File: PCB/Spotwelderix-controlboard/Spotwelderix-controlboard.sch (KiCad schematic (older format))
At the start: 45 parts, among them J1 LEDs, J2 ChargerPower, J3 ExtPwr_FAn, J4 Testpin, P1 Display, P2 CONN_01X08, Q1 AO3400A, Q2 AO3400A, Q3 AO3400A, U1 NodeMCU32, U2 LM7805M_TO263

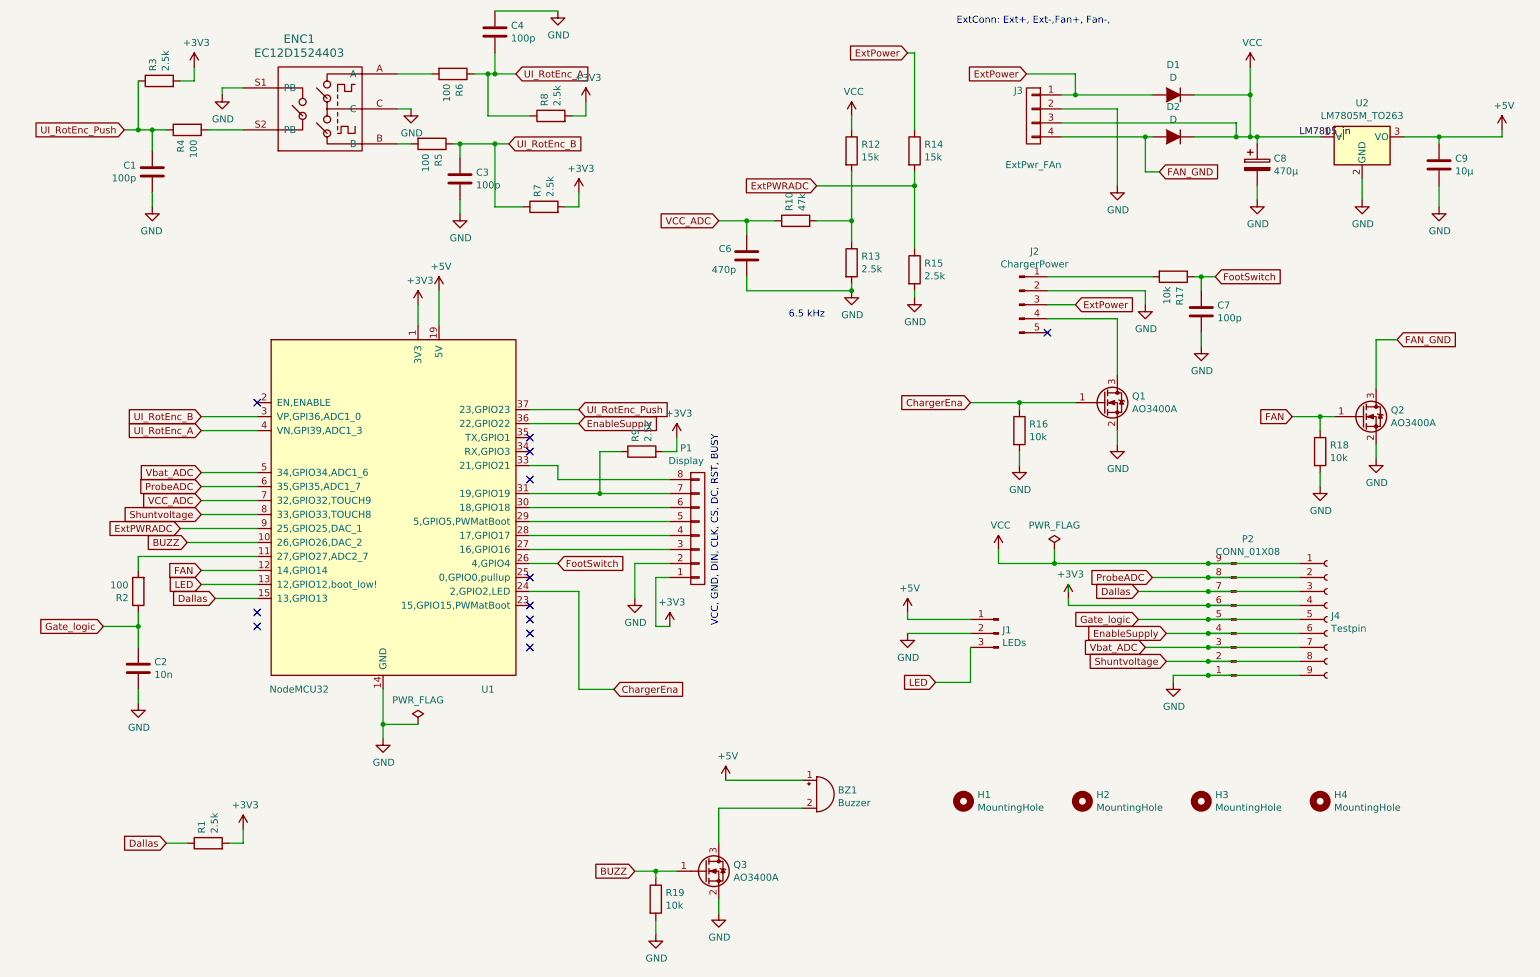
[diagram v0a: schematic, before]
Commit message: v3 commissioning
v3 has updated measurment devices to allow measurment of 1kA and voltages down to 0.3V accurately. Measeure the short!
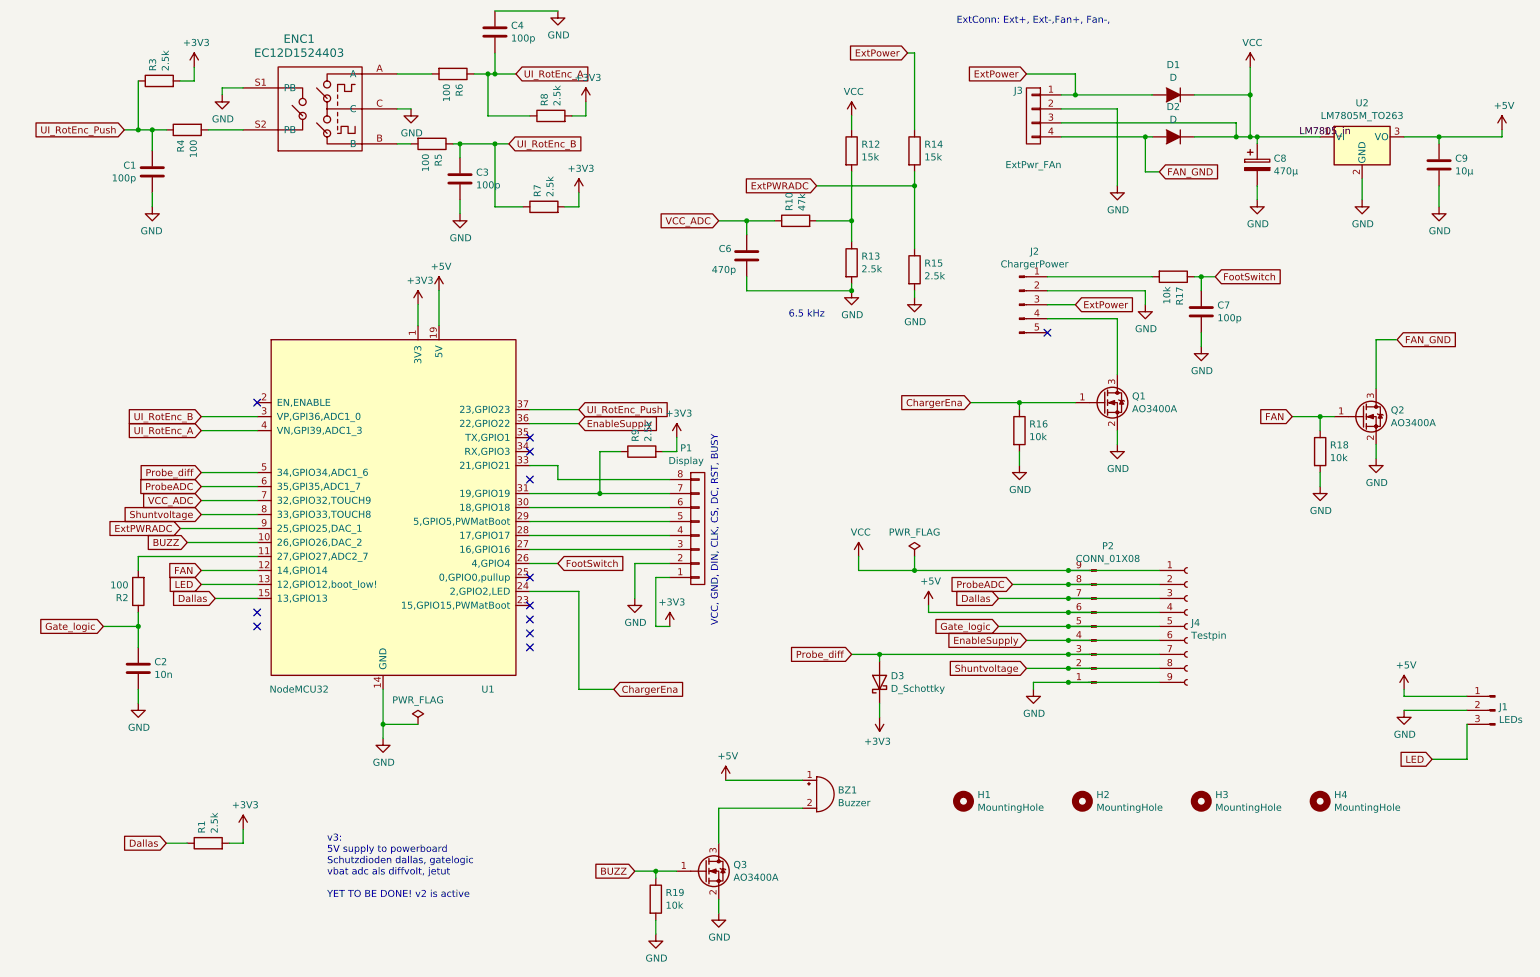
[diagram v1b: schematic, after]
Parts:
- added D3: D_Schottky, Diode_SMD:D_SMA_Handsoldering, symbol Device:D_Schottky
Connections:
- net +3V3: now also D3.1 (K); no longer J4.4 (Pin_4), P2.6 (Pin_6)
- net +5V: now also J4.4 (Pin_4), P2.6 (Pin_6)
- net Vbat_ADC renamed Probe_diff
- net Probe_diff: now also D3.2 (A)
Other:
- note added: "v3:\n5V supply to powerboard\nSchutzdioden dallas, gatelogic\nvbat adc als diffvolt, jetut\n\nYET TO BE DONE! v2 is active\n"
- moved on the sheet: J1, J4, P2
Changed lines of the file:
@@
 Title "Spotwelderix Controlboard"
 Date "2021-09-01"
-Rev "v02"
+Rev "v03"
 Comp ""
 Comment1 ""
@@
 Wire Wire Line
 	10150 3900 10150 3800
-Text GLabel 8450 4850 0    50   Input ~ 0
+Text GLabel 7450 4900 0    50   Input ~ 0
 Dallas
-Text GLabel 8650 5350 0    50   Input ~ 0
+Text GLabel 7650 5400 0    50   Input ~ 0
 Shuntvoltage
 $Comp
 L Spotwelderix-controlboard-rescue:GND-power #PWR029
 U 1 1 601723B2
-P 8700 5500
-F 0 "#PWR029" H 8700 5250 50  0001 C CNN
-F 1 "GND" H 8705 5327 50  0000 C CNN
-F 2 "" H 8700 5500 50  0001 C CNN
-F 3 "" H 8700 5500 50  0001 C CNN
-	1    8700 5500
-	1    0    0    -1
-$EndComp
-Wire Wire Line
-	8700 5500 8700 5450
-Text GLabel 8450 5050 0    50   Input ~ 0
+P 7700 5550
+F 0 "#PWR029" H 7700 5300 50  0001 C CNN
+F 1 "GND" H 7705 5377 50  0000 C CNN
+F 2 "" H 7700 5550 50  0001 C CNN
+F 3 "" H 7700 5550 50  0001 C CNN
+	1    7700 5550
+	1    0    0    -1
+$EndComp
+Wire Wire Line
+	7700 5550 7700 5500
+Text GLabel 7450 5100 0    50   Input ~ 0
 Gate_logic
-Wire Wire Line
-	7950 4800 7950 4850
 $Comp
 L Spotwelderix-controlboard-rescue:+5V-power #PWR09
@@
 L Spotwelderix-controlboard-rescue:Conn_01x03_Male-Connector J1
 U 1 1 6018AA6E
-P 7450 5150
-F 0 "J1" H 7422 5174 50  0000 R CNN
-F 1 "LEDs" H 7422 5083 50  0000 R CNN
-F 2 "Connector_JST:JST_XH_B3B-XH-A_1x03_P2.50mm_Vertical" H 7450 5150 50  0001 C CNN
-F 3 "~" H 7450 5150 50  0001 C CNN
-	1    7450 5150
+P 11000 5700
+F 0 "J1" H 10972 5724 50  0000 R CNN
+F 1 "LEDs" H 10972 5633 50  0000 R CNN
+F 2 "Connector_JST:JST_XH_B3B-XH-A_1x03_P2.50mm_Vertical" H 11000 5700 50  0001 C CNN
+F 3 "~" H 11000 5700 50  0001 C CNN
+	1    11000 5700
 	-1   0    0    -1
 $EndComp
@@
 L Spotwelderix-controlboard-rescue:GND-power #PWR021
 U 1 1 60191D79
-P 6800 5150
-F 0 "#PWR021" H 6800 4900 50  0001 C CNN
-F 1 "GND" H 6805 4977 50  0000 C CNN
-F 2 "" H 6800 5150 50  0001 C CNN
-F 3 "" H 6800 5150 50  0001 C CNN
-	1    6800 5150
+P 10350 5700
+F 0 "#PWR021" H 10350 5450 50  0001 C CNN
+F 1 "GND" H 10355 5527 50  0000 C CNN
+F 2 "" H 10350 5700 50  0001 C CNN
+F 3 "" H 10350 5700 50  0001 C CNN
+	1    10350 5700
 	1    0    0    -1
 $EndComp
@@
 L Spotwelderix-controlboard-rescue:+5V-power #PWR020
 U 1 1 60197CCB
-P 6800 5000
-F 0 "#PWR020" H 6800 4850 50  0001 C CNN
-F 1 "+5V" H 6815 5173 50  0000 C CNN
-F 2 "" H 6800 5000 50  0001 C CNN
-F 3 "" H 6800 5000 50  0001 C CNN
-	1    6800 5000
-	1    0    0    -1
-$EndComp
-Wire Wire Line
-	6800 5000 6800 5050
-Wire Wire Line
-	6800 5050 7250 5050
-Wire Wire Line
-	6800 5150 7250 5150
-Text GLabel 7000 5500 0    50   Input ~ 0
+P 10350 5550
+F 0 "#PWR020" H 10350 5400 50  0001 C CNN
+F 1 "+5V" H 10365 5723 50  0000 C CNN
+F 2 "" H 10350 5550 50  0001 C CNN
+F 3 "" H 10350 5550 50  0001 C CNN
+	1    10350 5550
+	1    0    0    -1
+$EndComp
+Wire Wire Line
+	10350 5550 10350 5600
+Wire Wire Line
+	10350 5600 10800 5600
+Wire Wire Line
+	10350 5700 10800 5700
+Text GLabel 10550 6050 0    50   Input ~ 0
 LED
 Wire Wire Line
-	7000 5500 7250 5500
-Wire Wire Line
-	7250 5500 7250 5250
+	10550 6050 10800 6050
+Wire Wire Line
+	10800 6050 10800 5800
 Text GLabel 1750 4800 0    50   Input ~ 0
 LED
@@
 	7900 1600 8500 1600
 Wire Wire Line
-	7450 4550 7450 4650
+	6450 4600 6450 4700
 Text GLabel 7650 1150 0    50   Input ~ 0
 ExtPower
@@
 $EndComp
 Wire Wire Line
-	8650 5150 8950 5150
-Wire Wire Line
-	8550 4750 8950 4750
-Wire Wire Line
-	8450 5050 8950 5050
-Wire Wire Line
-	8700 5450 8950 5450
+	7650 5200 7950 5200
+Wire Wire Line
+	7550 4800 7950 4800
+Wire Wire Line
+	7450 5100 7950 5100
+Wire Wire Line
+	7700 5500 7950 5500
 $Comp
 L Spotwelderix-controlboard-rescue:Conn_01x09_Male-Connector P2
 U 1 1 6015F832
-P 9150 5050
-F 0 "P2" H 9067 4475 50  0000 C CNN
-F 1 "CONN_01X08" H 9067 4566 50  0000 C CNN
-F 2 "Connector_JST:JST_XH_B9B-XH-A_1x09_P2.50mm_Vertical" H 9150 5050 50  0001 C CNN
-F 3 "" H 9150 5050 50  0000 C CNN
-	1    9150 5050
+P 8150 5100
+F 0 "P2" H 8067 4525 50  0000 C CNN
+F 1 "CONN_01X08" H 8067 4616 50  0000 C CNN
+F 2 "Connector_JST:JST_XH_B9B-XH-A_1x09_P2.50mm_Vertical" H 8150 5100 50  0001 C CNN
+F 3 "" H 8150 5100 50  0000 C CNN
+	1    8150 5100
 	-1   0    0    1
 $EndComp
 Wire Wire Line
-	8650 5350 8950 5350
-Text GLabel 8650 5150 0    50   Input ~ 0
+	7650 5400 7950 5400
+Text GLabel 7650 5200 0    50   Input ~ 0
 EnableSupply
-Text GLabel 8500 5250 0    50   Input ~ 0
-Vbat_ADC
 Text GLabel 1750 4100 0    50   Input ~ 0
 ProbeADC
@@
 VCC_ADC
 Text GLabel 1750 4000 0    50   Input ~ 0
-Vbat_ADC
+Probe_diff
 Text GLabel 1750 4300 0    50   Input ~ 0
 Shuntvoltage
@@
 Connection ~ 9250 1300
 Wire Wire Line
-	8500 5250 8950 5250
+	6400 5300 6600 5300
 Text GLabel 6800 1000 0    50   Input ~ 0
 ExtPower
@@
 L Spotwelderix-controlboard-rescue:VCC-power #PWR023
 U 1 1 602C9F87
-P 7450 4550
-F 0 "#PWR023" H 7450 4400 50  0001 C CNN
-F 1 "VCC" H 7465 4723 50  0000 C CNN
-F 2 "" H 7450 4550 50  0001 C CNN
-F 3 "" H 7450 4550 50  0001 C CNN
-	1    7450 4550
-	1    0    0    -1
-$EndComp
-Wire Wire Line
-	7450 4650 7850 4650
-Connection ~ 7850 4650
-Wire Wire Line
-	7850 4550 7850 4650
+P 6450 4600
+F 0 "#PWR023" H 6450 4450 50  0001 C CNN
+F 1 "VCC" H 6465 4773 50  0000 C CNN
+F 2 "" H 6450 4600 50  0001 C CNN
+F 3 "" H 6450 4600 50  0001 C CNN
+	1    6450 4600
+	1    0    0    -1
+$EndComp
+Wire Wire Line
+	6450 4700 6850 4700
+Connection ~ 6850 4700
+Wire Wire Line
+	6850 4600 6850 4700
 $Comp
 L Spotwelderix-controlboard-rescue:PWR_FLAG-power #FLG02
 U 1 1 602C3C21
-P 7850 4550
-F 0 "#FLG02" H 7850 4625 50  0001 C CNN
-F 1 "PWR_FLAG" H 7850 4723 50  0000 C CNN
-F 2 "" H 7850 4550 50  0001 C CNN
-F 3 "~" H 7850 4550 50  0001 C CNN
-	1    7850 4550
-	1    0    0    -1
-$EndComp
-$Comp
-L Spotwelderix-controlboard-rescue:+3V3-power #PWR025
-U 1 1 61300BA5
-P 7950 4900
-F 0 "#PWR025" H 7950 4750 50  0001 C CNN
-F 1 "+3V3" H 7965 5073 50  0000 C CNN
-F 2 "" H 7950 4900 50  0001 C CNN
-F 3 "" H 7950 4900 50  0001 C CNN
-	1    7950 4900
+P 6850 4600
+F 0 "#FLG02" H 6850 4675 50  0001 C CNN
+F 1 "PWR_FLAG" H 6850 4773 50  0000 C CNN
+F 2 "" H 6850 4600 50  0001 C CNN
+F 3 "~" H 6850 4600 50  0001 C CNN
+	1    6850 4600
 	1    0    0    -1
 $EndComp
@@
 L Connector:Conn_01x09_Female J4
 U 1 1 61345D7A
-P 9800 5050
-F 0 "J4" H 9828 5076 50  0000 L CNN
-F 1 "Testpin" H 9828 4985 50  0000 L CNN
-F 2 "Connector_PinHeader_2.54mm:PinHeader_1x09_P2.54mm_Vertical" H 9800 5050 50  0001 C CNN
-F 3 "~" H 9800 5050 50  0001 C CNN
-	1    9800 5050
-	1    0    0    -1
-$EndComp
-Wire Wire Line
-	7850 4650 8950 4650
-Connection ~ 8950 4650
-Wire Wire Line
-	8950 4650 9600 4650
-Wire Wire Line
-	8950 4750 9600 4750
-Connection ~ 8950 4750
-Wire Wire Line
-	9600 4850 8950 4850
-Wire Wire Line
-	8950 4950 9600 4950
-Connection ~ 8950 4950
-Wire Wire Line
-	9600 5050 8950 5050
-Connection ~ 8950 5050
-Wire Wire Line
-	8950 5150 9600 5150
-Connection ~ 8950 5150
-Wire Wire Line
-	8950 5250 9600 5250
-Connection ~ 8950 5250
-Wire Wire Line
-	9600 5350 8950 5350
-Connection ~ 8950 5350
-Wire Wire Line
-	8950 5450 9600 5450
-Connection ~ 8950 5450
-Wire Wire Line
-	7950 4900 7950 4950
-Wire Wire Line
-	7950 4950 8950 4950
-Wire Wire Line
-	8450 4850 8950 4850
-Connection ~ 8950 4850
+P 8800 5100
+F 0 "J4" H 8828 5126 50  0000 L CNN
+F 1 "Testpin" H 8828 5035 50  0000 L CNN
+F 2 "Connector_PinHeader_2.54mm:PinHeader_1x09_P2.54mm_Vertical" H 8800 5100 50  0001 C CNN
+F 3 "~" H 8800 5100 50  0001 C CNN
+	1    8800 5100
+	1    0    0    -1
+$EndComp
+Wire Wire Line
+	6850 4700 7950 4700
+Connection ~ 7950 4700
+Wire Wire Line
+	7950 4700 8600 4700
+Wire Wire Line
+	7950 4800 8600 4800
+Connection ~ 7950 4800
+Wire Wire Line
+	8600 4900 7950 4900
+Wire Wire Line
+	7950 5000 8600 5000
+Connection ~ 7950 5000
+Wire Wire Line
+	8600 5100 7950 5100
+Connection ~ 7950 5100
+Wire Wire Line
+	7950 5200 8600 5200
+Connection ~ 7950 5200
+Wire Wire Line
+	7950 5300 8600 5300
+Connection ~ 7950 5300
+Wire Wire Line
+	8600 5400 7950 5400
+Connection ~ 7950 5400
+Wire Wire Line
+	7950 5500 8600 5500
+Connection ~ 7950 5500
+Wire Wire Line
+	6950 4950 6950 5000
+Wire Wire Line
+	6950 5000 7950 5000
+Wire Wire Line
+	7450 4900 7950 4900
+Connection ~ 7950 4900
 $Comp
 L Arduino_Spot_Welderparts:R R2
@@
 Wire Wire Line
 	3800 1150 3700 1150
-Text GLabel 8550 4750 0    50   Input ~ 0
+Text GLabel 7550 4800 0    50   Input ~ 0
 ProbeADC
 $Comp
@@
 Wire Wire Line
 	9300 1600 9750 1600
+Text GLabel 6400 5300 0    50   Input ~ 0
+Probe_diff
+Text Notes 2650 7050 0    50   ~ 0
+v3:\n5V supply to powerboard\nSchutzdioden dallas, gatelogic\nvbat adc als diffvolt, jetut\n\nYET TO BE DONE! v2 is active\n
+$Comp
+L Spotwelderix-controlboard-rescue:+5V-power #PWR025
+U 1 1 62405CB9
+P 6950 4950
+F 0 "#PWR025" H 6950 4800 50  0001 C CNN
+F 1 "+5V" H 6965 5123 50  0000 C CNN
+F 2 "" H 6950 4950 50  0001 C CNN
+F 3 "" H 6950 4950 50  0001 C CNN
+	1    6950 4950
+	1    0    0    -1
+$EndComp
+$Comp
+L Device:D_Schottky D3
+U 1 1 62443536
+P 6600 5500
+F 0 "D3" V 6646 5420 50  0000 R CNN
+F 1 "D_Schottky" V 6555 5420 50  0000 R CNN
+F 2 "Diode_SMD:D_SMA_Handsoldering" H 6600 5500 50  0001 C CNN
+F 3 "~" H 6600 5500 50  0001 C CNN
+	1    6600 5500
+	0    -1   -1   0
+$EndComp
+$Comp
+L Spotwelderix-controlboard-rescue:+3V3-power #PWR017
+U 1 1 62444B82
+P 6600 5750
+F 0 "#PWR017" H 6600 5600 50  0001 C CNN
+F 1 "+3V3" H 6615 5923 50  0000 C CNN
+F 2 "" H 6600 5750 50  0001 C CNN
+F 3 "" H 6600 5750 50  0001 C CNN
+	1    6600 5750
+	-1   0    0    1
+$EndComp
+Wire Wire Line
+	6600 5750 6600 5650
+Wire Wire Line
+	6600 5350 6600 5300
+Connection ~ 6600 5300
+Wire Wire Line
+	6600 5300 7950 5300
 $EndSCHEMATC
